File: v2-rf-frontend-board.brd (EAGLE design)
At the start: 85.7 x 40.9 mm, 151 parts, among them J1 USB_MICROB, J2 MICROSD, J3 ROCKETNET-CONNECTOR-16M, Q1 NTR4101P, T1 ALT4532, T2 ALT4532, U1 MAX2769, U2 SAW, U3 LAN8710A-EZC, U4 7Q-16.368MBG-T, U5 XC2401, U7 LT4619_REDUCED, U8 STM32F4V, U9 LM3480IM4, X1 25 MHz, X2 BU-SMA-H

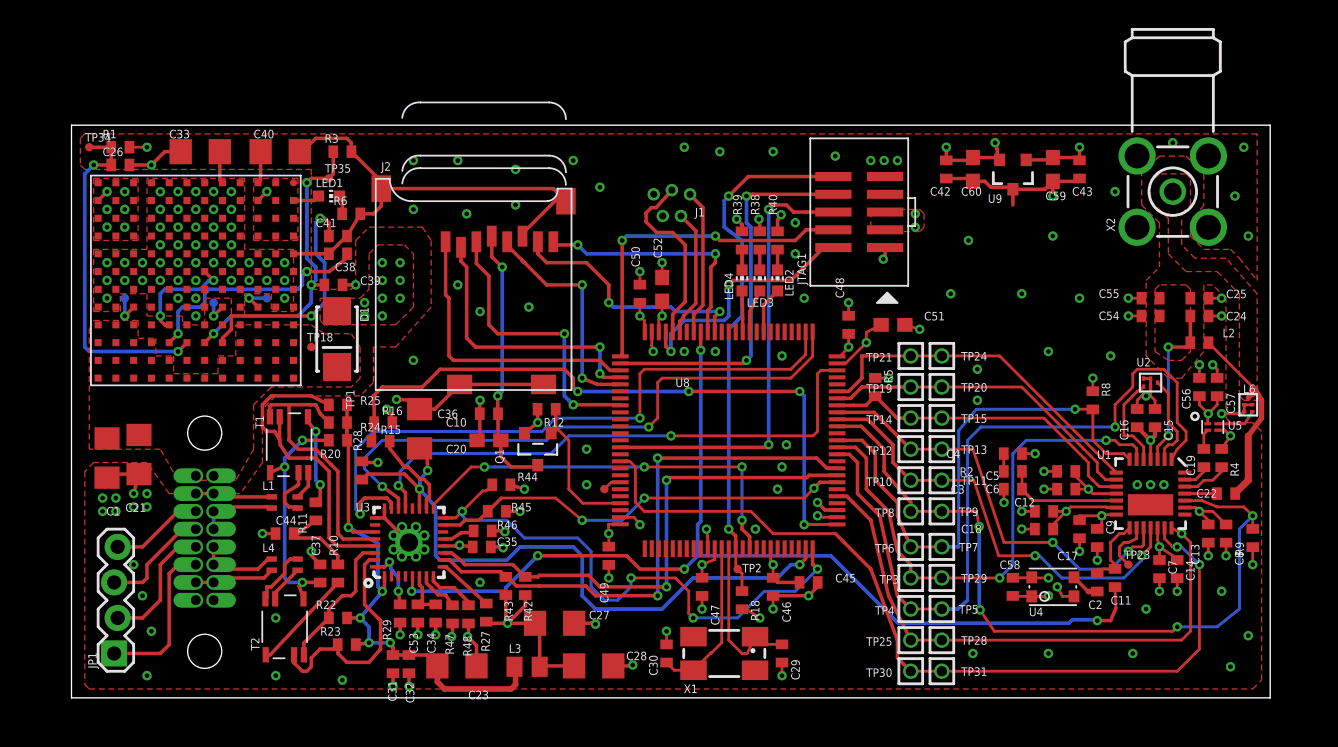
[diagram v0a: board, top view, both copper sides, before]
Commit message: Fixes as per design review. microUSB footprint needs help but symbol and signals OK. RF side placement adjusted but impedance 50 ohms wants 14mm wide trace. help.
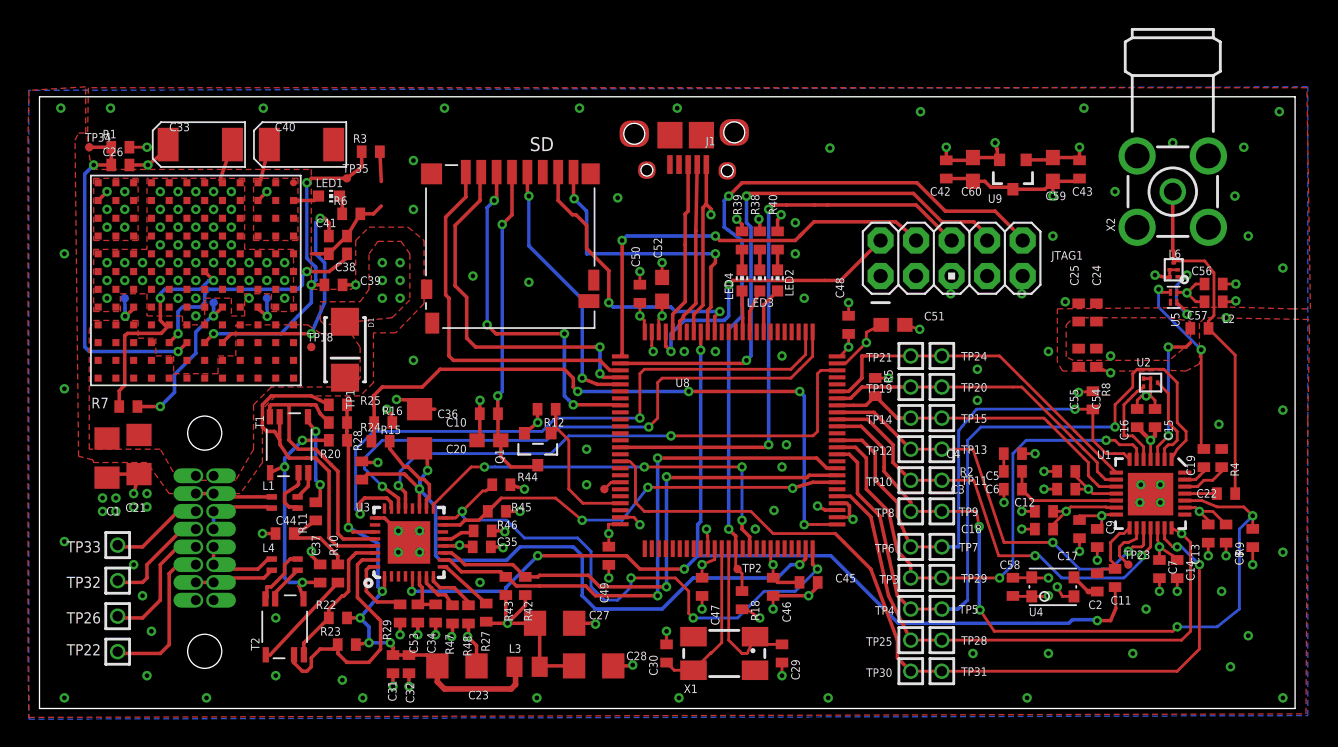
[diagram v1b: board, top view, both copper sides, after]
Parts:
- removed J2: MICROSD, adafruit:MICROSD
- removed JP1: AUX HDR, SparkFun-Connectors:1X04_LOCK
- added R7: 100k, rcl:R0402
- added SD: CON_HIROSE_DM3D(MICROSD), con-usd-hirose-dm3-gpsboard:HIROSE_DM3D(MICRO-SD)
- added TP22, TP26, TP32, TP33: TEST-POINT, Tova:2MM-TEST-POINT
- C33, C40: device rcl:C1206 -> SparkFun-Passives:EIA6032
- J1: device SparkFun:MICRO-B-RA-TH -> con-hirose-microusb:ZX62D-B-5P8
- JTAG1: value (none) -> M05X2PTH; device microbuilder:2X05_1.27MM_SMT -> SparkFun-Connectors:AVR_ICSP
- U9: value LM3480IM4 -> LM3480IM3
- moved L6 11.0 mm to (78.8, 30.6)
- moved U5 9.68 mm to (78.8, 28.6), turned to 180 degrees
- moved C25 8.70 mm to (72.0, 27.6), turned to 90 degrees
- moved C56 7.44 mm to (81.7, 29.6), turned to 0 degrees
- moved JTAG1 7.38 mm to (62.9, 31.4)
- moved C24 7.37 mm to (73.3, 27.6), turned to 90 degrees
- moved C55 6.68 mm to (72.0, 24.3), turned to 270 degrees
- moved C57 6.10 mm to (81.7, 28.3), turned to 0 degrees
- moved J1 5.14 mm to (43.7, 40.1)
- moved C54 4.89 mm to (73.3, 24.3), turned to 270 degrees
- moved R3 2.03 mm to (21.4, 39.1)
- moved C40 1.61 mm to (16.4, 39.6)
- moved TP35 1.27 mm to (19.7, 37.1)
- moved L2 1.02 mm to (80.6, 26.4)
- moved D1 0.95 mm to (19.6, 24.9)
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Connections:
- removed net N$4: TP27.TP, U7.H5
- removed net N$46: J3.A1, JP1.1
- removed net N$47: J3.A2, JP1.2
- removed net N$48: J3.A3, JP1.3
- removed net N$50: J3.A4, JP1.4
- new net AUX1: J3.A1, TP22.1
- new net AUX2: J3.A2, TP26.1
- new net AUX3: J3.A3, TP32.1
- new net AUX4: J3.A4, TP33.1
- new net PGOOD: R7.1, TP27.TP, U7.H5
- net +5V: now also C33.P$1; no longer C33.1
- net 3.3VD: now also C40.P$1; no longer C40.1
- net GND: now also C33.P$2, C40.P$2, J1.G1, J1.G2, J1.G3, J1.G4, J1.G5, J1.G6, J1.P5, SD.G1, SD.G2, SD.G3, SD.G4, SD.P6, SD.S0, SD.S1, U3.GND, U8.PA4; no longer C33.2, C40.2, J1.5, J2.6, J2.CD1, J2.CD2, J2.MT1, J2.MT2, U3.EP1, U3.EP2, U3.EP3, U3.EP4, U3.EP5, U3.EP6, U3.EP7, U3.EP8, U3.EP9
- net N$6: now also R7.2
- net OTG_FS_DM: now also J1.P2; no longer J1.2
- net OTG_FS_DP: now also J1.P3; no longer J1.3
- net OTG_FS_VBUS: now also J1.P1; no longer J1.1
- net SDIO_CLK: now also SD.P5; no longer J2.5
- net SDIO_CMD: now also SD.P3; no longer J2.3
- net SDIO_D0: now also SD.P7; no longer J2.7
- net SDIO_D1: now also SD.P8; no longer J2.8
- net SDIO_D2: now also SD.P1; no longer J2.1
- net SDIO_D3: now also SD.P2; no longer J2.2
- net VDD: now also SD.P4; no longer J2.4
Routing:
- net GND: track 141.4 -> 101.4 mm, vias 175 -> 187
- net !RST: track 37.9 -> 53.0 mm
- net TDI: track 27.4 -> 40.2 mm
- net LNA1: track 1.46 -> 13.7 mm, vias 0 -> 2
- net PGOOD: track 0.00 -> 11.6 mm, vias 0 -> 2
- net N$46: track 11.4 -> 0.00 mm
- net LNA2: track 13.8 -> 25.2 mm
- net AUX1: track 0.00 -> 11.2 mm
- net TDO: track 32.5 -> 41.8 mm
- net AUX2: track 0.00 -> 9.23 mm
- net N$47: track 9.18 -> 0.00 mm
- net VIN: track 0.00 -> 8.76 mm
- net N$6: track 7.77 -> 16.5 mm
- net N$48: track 7.98 -> 0.00 mm
- net AUX3: track 0.00 -> 7.78 mm
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- added copper zone on layer 15, net +5V
- added copper zone on layer 15, net 3.3VA
- added copper zone on layer 15, net 3.3VD
- added copper zone on layer 16, net GND
- added copper zone on layer 2, net GND
- added copper zone on layer 15, net OTG_FS_VBUS
- removed copper zone on layer 2, net +5V
- removed copper zone on layer 2, net 3.3VA
- removed copper zone on layer 2, net 3.3VD
- removed copper zone on layer 1, net LNA2
- removed copper zone on layer 2, net OTG_FS_VBUS
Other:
- board size 85.7 x 40.9 mm -> 89.8 x 43.7 mm
